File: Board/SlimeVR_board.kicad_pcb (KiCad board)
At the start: 2 copper layers, 55.8 x 44.5 mm, 44 parts, among them IC1 HT7833, J1 USB_C_Receptacle_USB2.0_16P, J2 Conn_01x02_Pin, J3 Conn_01x04_Pin, J5 Conn_01x01_Pin, J6 Conn_01x01_Pin, J7 Conn_01x04_Pin, Q1 DMP3099L, SW1 SW_SPDT, U1 TP4056-42-ESOP8, U2 ESP32-C3-WROOM-02

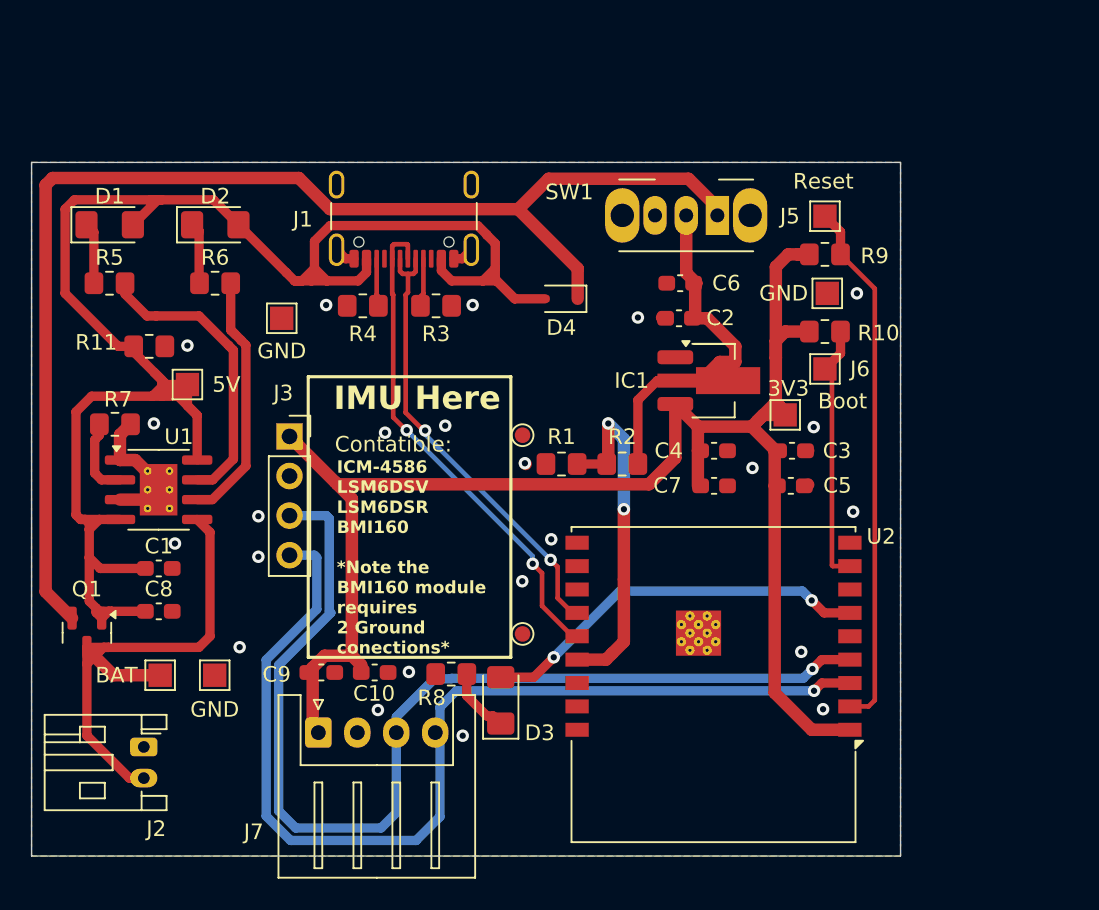
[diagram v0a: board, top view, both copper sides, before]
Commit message: New Version
skiped few version that ware bad or not good or not funcioning
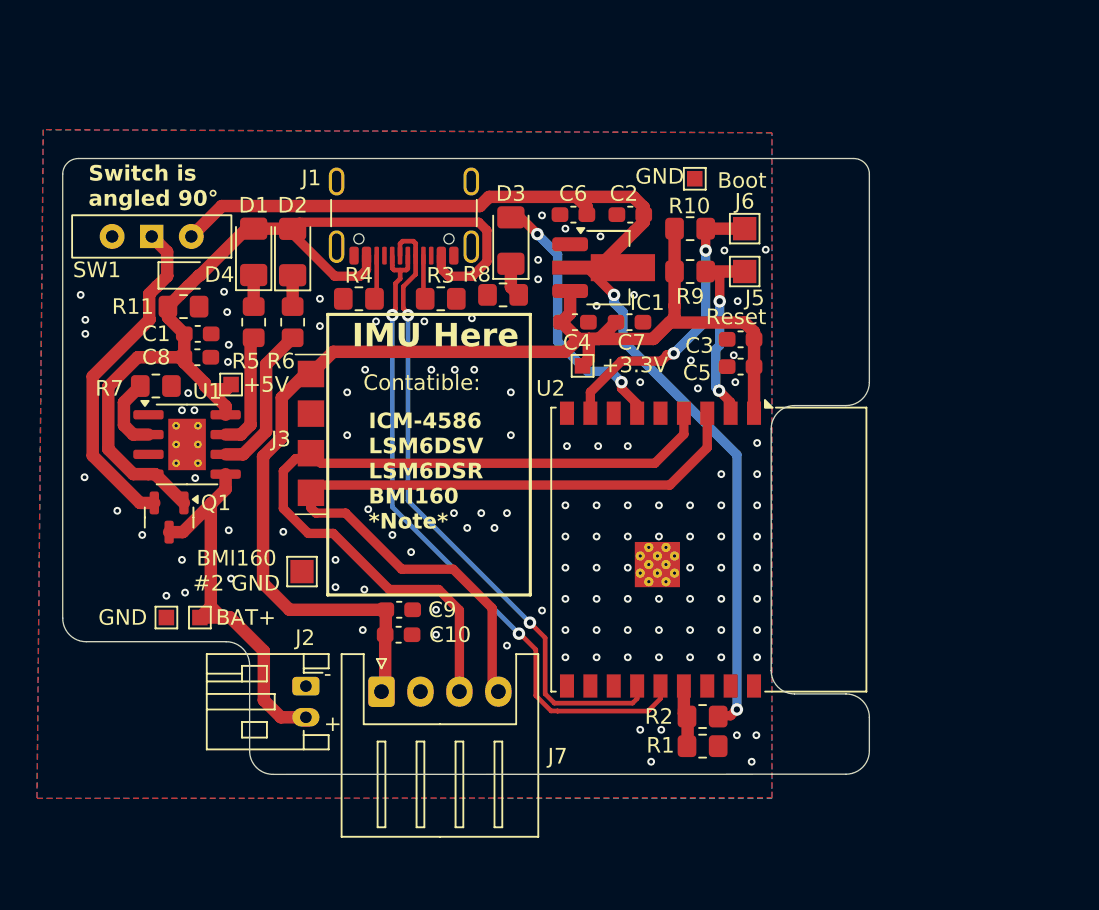
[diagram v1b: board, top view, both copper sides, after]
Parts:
- removed 3V3, 5V, BAT: TestPoint_Pad_1.5x1.5mm, TestPoint:TestPoint_Pad_1.5x1.5mm
- removed the GND at (82.3, 34.4)
- removed the GND at (47.3, 36.0)
- removed the GND at (43.0, 58.9)
- removed REF** (x2): TestPoint_Pad_D1.0mm, TestPoint:TestPoint_Pad_D1.0mm
- added +3.3V: TestPoint_Pad_1.0x1.0mm, TestPoint:TestPoint_Pad_1.0x1.0mm, F.Cu at (66.6, 39.0)
- added +5V: TestPoint_Pad_1.0x1.0mm, TestPoint:TestPoint_Pad_1.0x1.0mm, F.Cu at (44.0, 40.2)
- added BAT+: TestPoint_Pad_1.0x1.0mm, TestPoint:TestPoint_Pad_1.0x1.0mm, F.Cu at (42.0, 55.2)
- added BMI160 #2 GND: TestPoint_Pad_1.5x1.5mm, TestPoint:TestPoint_Pad_1.5x1.5mm, F.Cu at (48.6, 52.2)
- added GND: TestPoint_Pad_1.0x1.0mm, TestPoint:TestPoint_Pad_1.0x1.0mm, F.Cu at (39.9, 55.2)
- added GND: TestPoint_Pad_1.0x1.0mm, TestPoint:TestPoint_Pad_1.0x1.0mm, F.Cu at (73.8, 27.1)
- D1: value LED -> FYLS-1206URC
- D2: value LED -> FYLS-1206PGC
- D3: value LED -> FYLS-1206UWC
- D4: value D -> 1N4148WSQ-7-F
- J2: value Conn_01x02_Pin -> JST-PH
- J3: value Conn_01x04_Pin -> SMD_Pads; footprint Connector_PinSocket_2.54mm:PinSocket_1x04_P2.54mm_Vertical -> Custom:Pin_1x04_SMD_P2.54mm
- J7: value Conn_01x04_Pin -> JTX-HX
- Q1: value DMP3099L -> DMP3099L-7
- R1: value 10k -> 47k
- R2: value 3k3 -> 47k
- SW1: value SW_SPDT -> LA215009; footprint Button_Switch_THT:SW_Slide_SPDT_Angled_CK_OS102011MA1Q -> Button_Switch_THT:SW_Slide-03_Wuerth-WS-SLTV_10x2.5x6.4_P2.54mm
- moved SW1 36.3 mm to (39.0, 30.8)
- moved D3 29.5 mm to (62.0, 31.0)
- moved R8 24.6 mm to (61.5, 34.5)
- moved D4 24.3 mm to (41.0, 33.2), turned to 0 degrees
- moved R1 20.2 mm to (74.3, 63.5), turned to 0 degrees
- moved R2 17.0 mm to (74.3, 61.5)
- moved C8 16.5 mm to (41.9, 38.5)
- moved C1 15.3 mm to (41.9, 37.0)
- moved C4 12.2 mm to (66.1, 36.2)
- moved C7 11.8 mm to (69.6, 36.2)
- moved J2 11.1 mm to (48.9, 59.6)
- moved R10 10.9 mm to (73.5, 30.2)
- moved J6 10.4 mm to (77.0, 30.2)
- moved IC1 9.91 mm to (68.2, 32.8)
- moved R5 9.58 mm to (45.5, 36.2), turned to -90 degrees
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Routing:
- net Net-(D4-K): track 82.0 -> 21.7 mm
- net +5V: track 117.3 -> 62.9 mm
- net Net-(SW1-B): track 22.6 -> 74.0 mm, vias 0 -> 2
- net +3.3V: track 103.9 -> 80.0 mm
- net Net-(J5-Pin_1): track 34.1 -> 12.8 mm, vias 0 -> 2
- net Net-(U2-IO3): track 22.4 -> 4.09 mm, vias 2 -> 0
- net Net-(J3-Pin_3): track 68.0 -> 50.2 mm, vias 1 -> 0
- net Net-(J3-Pin_4): track 66.1 -> 49.6 mm, vias 1 -> 0
- net D-: track 29.4 -> 42.0 mm
- net Earth: track 12.2 -> 0.00 mm, vias 23 -> 117
- net D+: track 32.1 -> 43.6 mm
- net Net-(U1-~{CHRG}): track 19.0 -> 7.53 mm
- net Net-(D3-A): track 25.6 -> 17.2 mm
- net +BATT: track 33.9 -> 26.3 mm
- net Net-(U1-~{STDBY}): track 17.0 -> 9.92 mm
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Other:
- board size 55.8 x 44.5 mm -> 51.8 x 39.5 mm
- board text added: "*Note: for BMI160 bridge bouth GNDs as show in SlimeVR Documentation*"
- board text added: "+3V3"
- board text added: "- +"
- board text added: "GND"
- board text added: "ICM-4586 LSM6DSV LSM6DSR BMI160 *Note*"
- board text added: "None"
- board text added: "Powered \/ \/"
- board text added: "SCl"
- board text added: "SDA"
- board text added: "Switch is angled 90°"
- board text added: "Ver.: 0.9C"
- board text removed: "ICM-4586 LSM6DSV LSM6DSR BMI160 *Note the BMI160 module requires 2 Ground conections*"

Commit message: New version
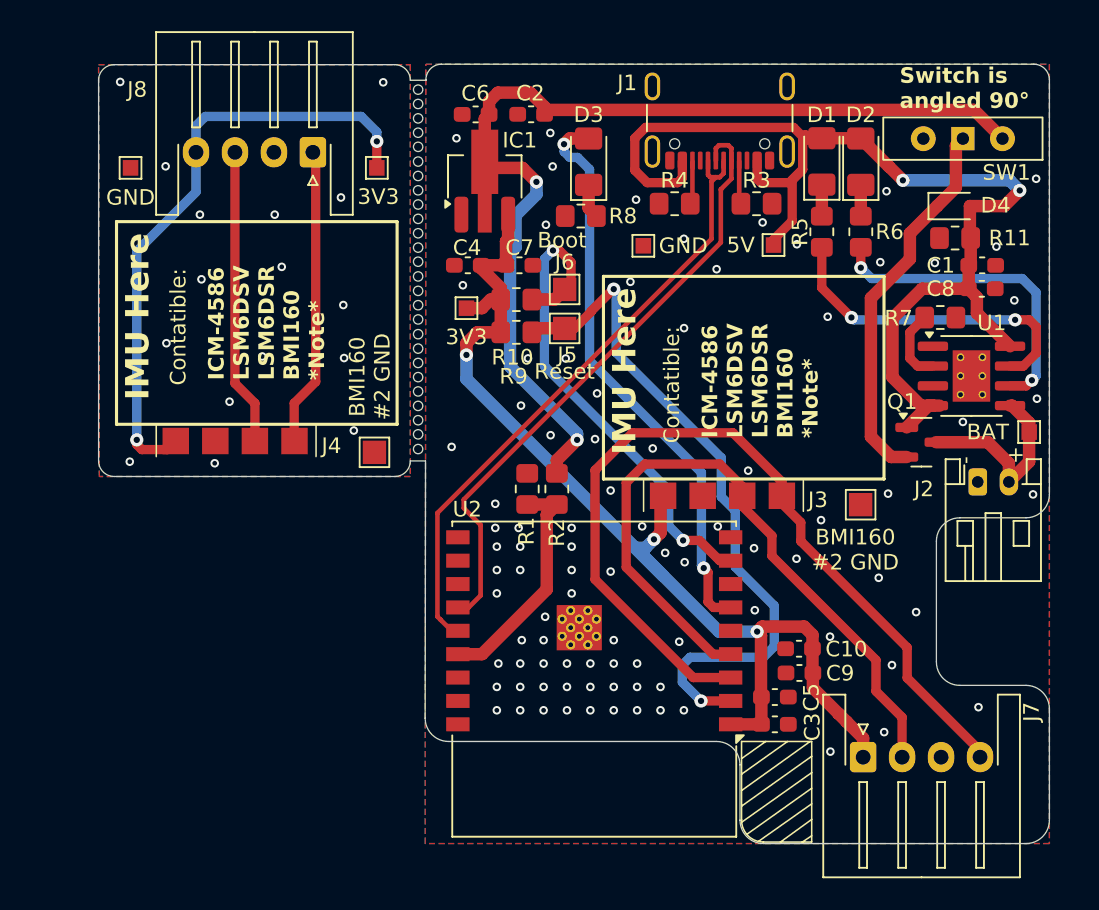
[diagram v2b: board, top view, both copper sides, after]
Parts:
- removed +3.3V, +5V, BAT+: TestPoint_Pad_1.0x1.0mm, TestPoint:TestPoint_Pad_1.0x1.0mm
- removed the GND at (39.9, 55.2)
- removed the GND at (73.8, 27.1)
- added 3V3: TestPoint_Pad_1.0x1.0mm, TestPoint:TestPoint_Pad_1.0x1.0mm, F.Cu at (53.4, 26.4)
- added 3V3: TestPoint_Pad_1.0x1.0mm, TestPoint:TestPoint_Pad_1.0x1.0mm, F.Cu at (59.1, 35.4)
- added 5V: TestPoint_Pad_1.0x1.0mm, TestPoint:TestPoint_Pad_1.0x1.0mm, F.Cu at (78.8, 31.3)
- added BAT: TestPoint_Pad_1.0x1.0mm, TestPoint:TestPoint_Pad_1.0x1.0mm, F.Cu at (95.2, 43.3)
- added BMI160 #2 GND: TestPoint_Pad_1.5x1.5mm, TestPoint:TestPoint_Pad_1.5x1.5mm, F.Cu at (53.2, 44.6)
- added GND: TestPoint_Pad_1.0x1.0mm, TestPoint:TestPoint_Pad_1.0x1.0mm, F.Cu at (37.6, 26.4)
- added GND: TestPoint_Pad_1.0x1.0mm, TestPoint:TestPoint_Pad_1.0x1.0mm, F.Cu at (70.5, 31.4)
- added J4: SMD_Pads, Custom:Pin_1x04_SMD_P2.54mm, F.Cu at (45.0, 46.4)
- added J8: JTX-HX-A-1, Connector_JST:JST_XH_S4B-XH-A-1_1x04_P2.50mm_Horizontal, F.Cu at (49.3, 25.4)
- J7: value JTX-HX -> JTX-HX-A-1; footprint Connector_JST:JST_XH_S4B-XH-A_1x04_P2.50mm_Horizontal -> Connector_JST:JST_XH_S4B-XH-A-1_1x04_P2.50mm_Horizontal
- U1: value TP4056-42-ESOP8 -> TP4056-ESOP8
- U2: value ESP32-C3-WROOM-02 -> ESP32-C3-WROOM-02-N4
- moved SW1 52.4 mm to (91.0, 24.5)
- moved C8 50.5 mm to (92.2, 34.1)
- moved C1 50.5 mm to (92.2, 32.6)
- moved R7 50.5 mm to (89.5, 36.0)
- moved U1 50.5 mm to (91.5, 39.7)
- moved R11 49.7 mm to (90.5, 30.9), turned to 0 degrees
- moved D4 49.6 mm to (90.4, 28.8)
- moved Q1 48.5 mm to (88.3, 44.0), turned to 0 degrees
- moved J2 45.0 mm to (92.0, 46.5), turned to 0 degrees
- moved D1 36.9 mm to (82.0, 25.9)
- moved D2 36.9 mm to (84.5, 25.9)
- moved R5 36.9 mm to (82.0, 30.4)
- moved R6 36.9 mm to (84.5, 30.4)
- moved BMI160 #2 GND 36.1 mm to (84.4, 48.0), turned to 90 degrees
- moved J7 31.2 mm to (84.6, 64.2)
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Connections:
- net Net-(J3-Pin_4) renamed SDA
- net Net-(U2-IO3) renamed Battery_sence
- J3 pad 3: Net-(J3-Pin_3) -> SCL
- J7 pad 2: Earth -> SCL
- J7 pad 3: Net-(J3-Pin_3) -> Earth
- U2 pad 4: Net-(J3-Pin_3) -> SCL
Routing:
- net SCL: track 0.00 -> 63.6 mm
- net Net-(J3-Pin_3): track 50.2 -> 0.00 mm
- net Net-(J5-Pin_1): track 12.8 -> 45.1 mm
- net +3.3V: track 80.0 -> 109.9 mm, vias 0 -> 5
- net SDA: track 49.6 -> 74.7 mm
- net Net-(D3-A): track 17.2 -> 36.8 mm
- net +BATT: track 26.3 -> 12.5 mm
- net Net-(U1-~{CHRG}): track 7.53 -> 21.1 mm, vias 0 -> 2
- net Net-(J6-Pin_1): track 19.1 -> 31.9 mm
- net +5V: track 62.9 -> 75.6 mm, vias 0 -> 2
- net Battery_sence: track 4.09 -> 15.0 mm
- net Net-(U1-~{STDBY}): track 9.92 -> 20.5 mm, vias 0 -> 2
- net Net-(SW1-B): track 74.0 -> 70.2 mm
- net D+: track 43.6 -> 40.2 mm, vias 2 -> 0
- net Net-(D4-K): track 21.7 -> 24.4 mm
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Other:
- board size 51.8 x 39.5 mm -> 61 x 50 mm
- board text added: "Ver.: 2.5W"
- board text added: "Ver.: 2.5WE"
- board text added: "©2025 Skaut0071"
- board text removed: "Ver.: 0.9C"
